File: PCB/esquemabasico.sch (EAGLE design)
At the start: 10 parts

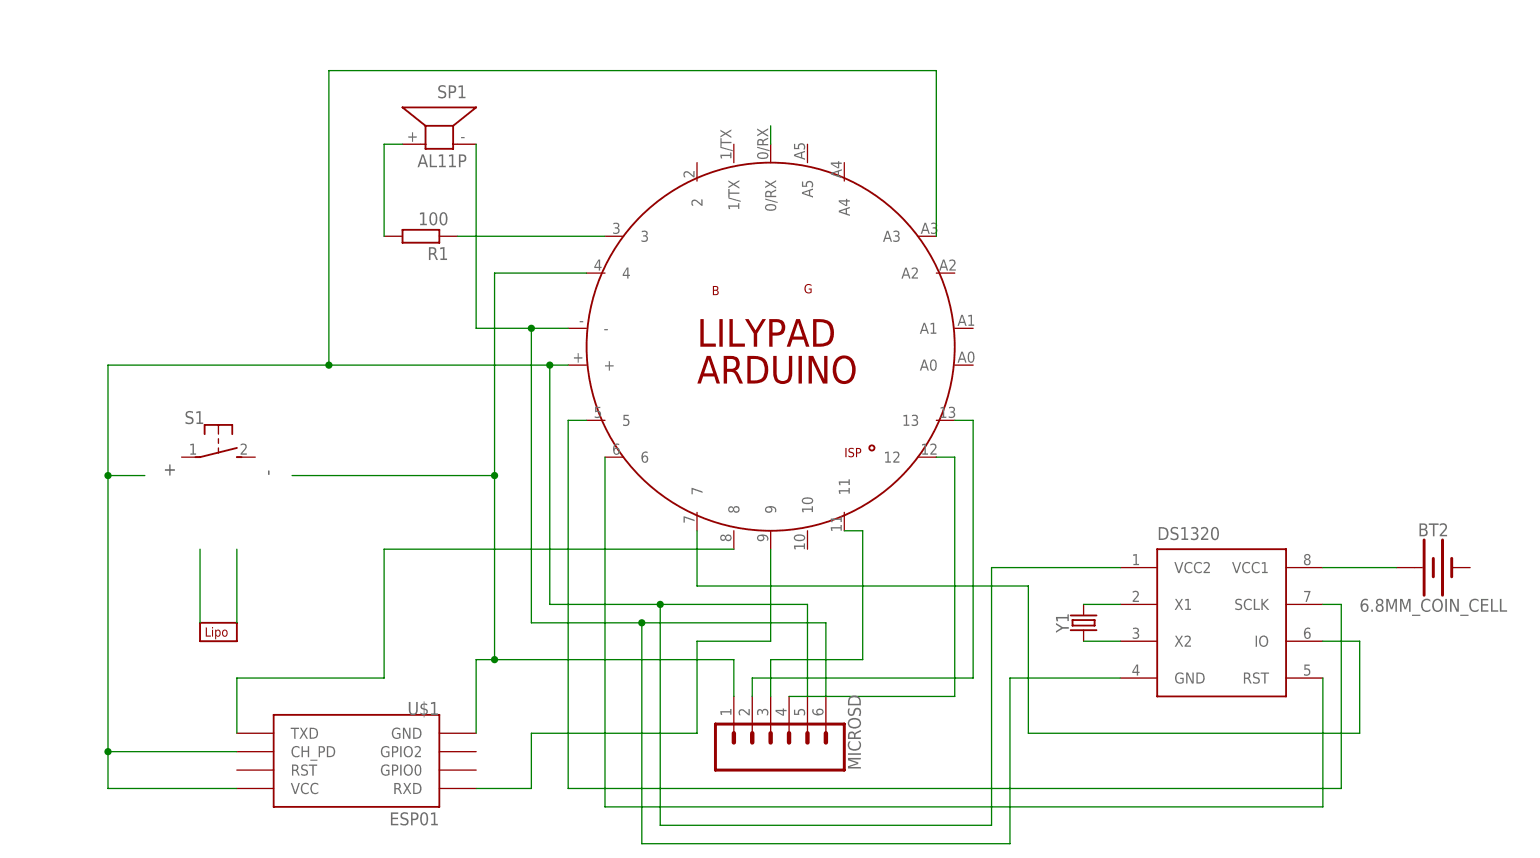
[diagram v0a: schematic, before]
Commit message: Cambios Finales PCB
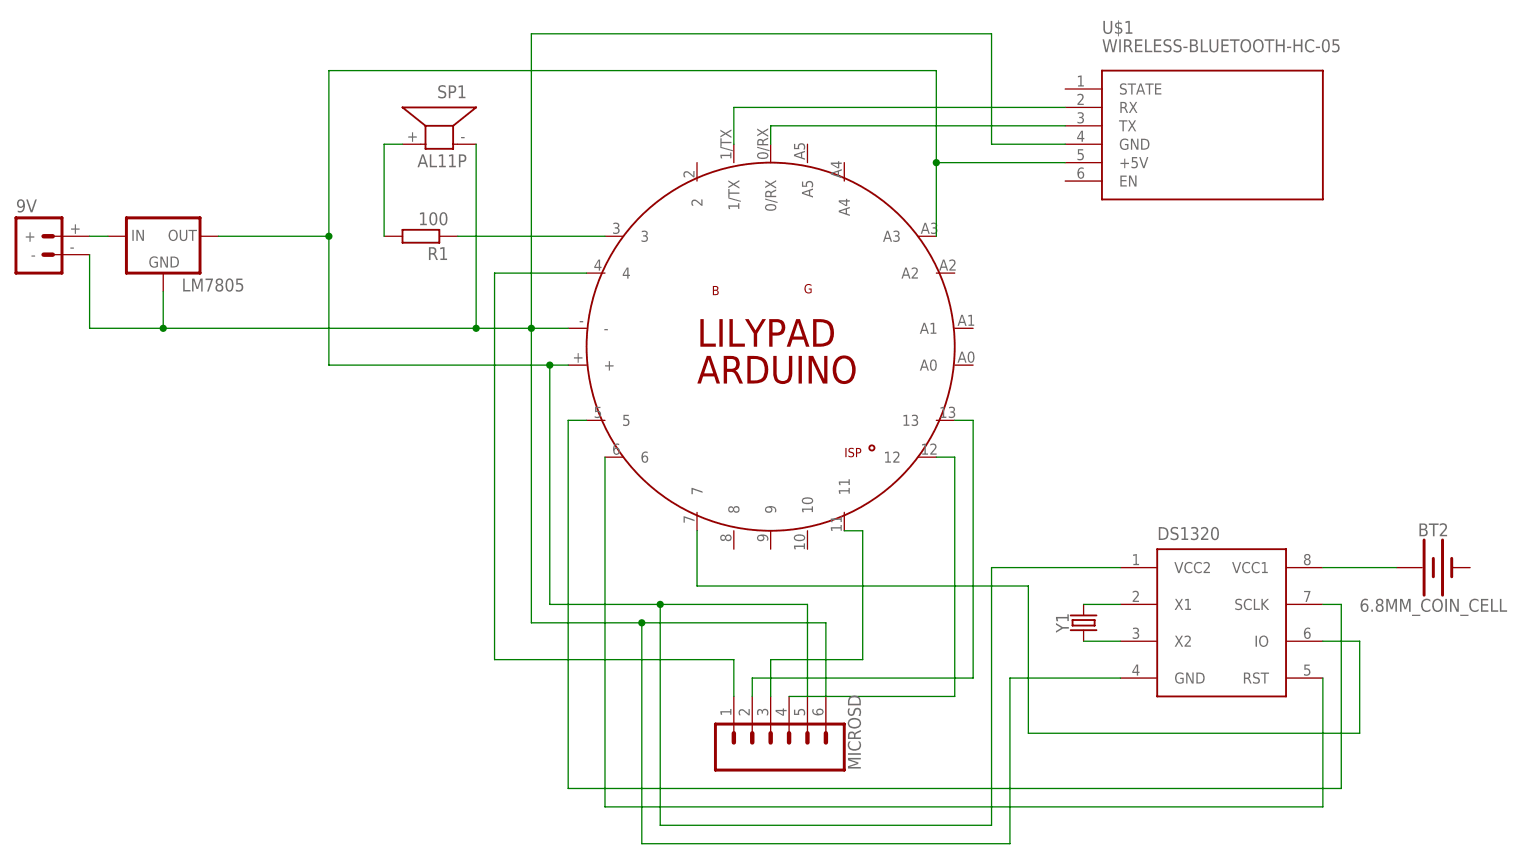
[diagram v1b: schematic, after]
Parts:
- removed BT1: LIPO-OUTLINE1100, SparkFun-Batteries:LIPO-OUTLINE1100
- removed S1: (no value), switch-omron:31-XX
- added 9V: (no value), SparkFun-Connectors:BATTERY_CONN_DEANS
- added LM7805: (no value), SparkFun-IC-Power:V_REG_78XX-TO-220
- U$1: value ESP01 -> WIRELESS-BLUETOOTH-HC-05; device esp8266:ESP01 -> diy-modules:WIRELESS-BLUETOOTH-HC-05
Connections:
- removed net N$19: PCB1.9, U$1.RXD
- new net N$2: 9V.+, LM7805.IN
- new net N$6: PCB1.1/TX, U$1.RX
- net N$1: no longer U$1.GND
- net N$14: now also U$1.TX
- net N$17: now also U$1.GND; no longer PCB1.8, U$1.TXD
- net N$3: now also LM7805.OUT, U$1.+5V; no longer U$1.CH_PD, U$1.VCC
- net N$5: now also 9V.-, LM7805.GND
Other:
- note removed: "+"
- note removed: "-"
- note removed: "Lilypad Simple Power"
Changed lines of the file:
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@@
 <part name="SP1" library="buzzer" library_urn="urn:adsk.eagle:library:113" deviceset="AL11P" device="" package3d_urn="urn:adsk.eagle:package:5308/1"/>
 <part name="R1" library="rcl" library_urn="urn:adsk.eagle:library:334" deviceset="R-EU_" device="0309/12" package3d_urn="urn:adsk.eagle:package:23571/1" value="100"/>
-<part name="BT1" library="SparkFun-Batteries" deviceset="LIPO-OUTLINE" device="1100"/>
-<part name="S1" library="switch-omron" library_urn="urn:adsk.eagle:library:377" deviceset="31-XX" device="" package3d_urn="urn:adsk.eagle:package:27487/1"/>
 <part name="DS1320" library="ltc1440_lt1529_ds1302" deviceset="DS1302" device=""/>
 <part name="BT2" library="SparkFun-Batteries" deviceset="BATTERY" device="-6.8MM_SMD" value="6.8MM_COIN_CELL"/>
 <part name="Y1" library="SparkFun-Clocks" deviceset="CRYSTAL" device="PTH-2X6"/>
-<part name="U$1" library="esp8266" deviceset="ESP01" device=""/>
+<part name="LM7805" library="SparkFun-IC-Power" deviceset="V_REG_78XX" device="-TO-220"/>
+<part name="9V" library="SparkFun-Connectors" deviceset="BATTERY_CONN" device="_DEANS"/>
+<part name="U$1" library="diy-modules" deviceset="WIRELESS-BLUETOOTH-HC-05" device=""/>
 </parts>
 <sheets>
 <sheet>
 <plain>
-<circle x="-12.7" y="25.4" radius="10.77630625" width="0.254" layer="133"/>
-<text x="-20.32" y="25.4" size="1.778" layer="97">+</text>
-<text x="-5.08" y="25.4" size="1.778" layer="97" rot="R90">-</text>
-<polygon width="0.254" layer="133" spacing="0.254" pour="hatch">
-<vertex x="-15.24" y="38.1"/>
-<vertex x="-15.24" y="35.56"/>
-<vertex x="-10.16" y="35.56"/>
-<vertex x="-10.16" y="38.1"/>
-</polygon>
-<text x="0" y="20.32" size="1.778" layer="133" rot="R180">Lilypad Simple Power</text>
 </plain>
 <instances>
@@
 <attribute name="VALUE" x="19.05" y="61.722" size="1.778" layer="96" rot="R180"/>
 </instance>
-<instance part="BT1" gate="G$1" x="-15.24" y="2.54" smashed="yes"/>
-<instance part="S1" gate="1" x="-12.7" y="27.94" smashed="yes" rot="R270">
-<attribute name="NAME" x="-14.605" y="34.29" size="1.778" layer="95" rot="R180"/>
-<attribute name="VALUE" x="-9.525" y="31.75" size="1.778" layer="96"/>
-</instance>
 <instance part="DS1320" gate="G$1" x="124.46" y="5.08" smashed="yes">
 <attribute name="NAME" x="116.84" y="16.51" size="1.778" layer="95"/>
@@
 <attribute name="VALUE" x="108.712" y="5.08" size="1.778" layer="96" font="vector" rot="R90" align="top-center"/>
 </instance>
-<instance part="U$1" gate="G$1" x="5.08" y="-17.78" smashed="yes" rot="MR0">
-<attribute name="NAME" x="17.78" y="-7.62" size="1.778" layer="95" rot="MR0"/>
-<attribute name="VALUE" x="17.78" y="-22.86" size="1.778" layer="95" rot="MR0"/>
+<instance part="LM7805" gate="G$1" x="-20.32" y="58.42" smashed="yes">
+<attribute name="NAME" x="-17.78" y="50.8" size="1.778" layer="95"/>
+<attribute name="VALUE" x="-17.78" y="48.26" size="1.778" layer="96"/>
+</instance>
+<instance part="9V" gate="G$1" x="-38.1" y="58.42" smashed="yes">
+<attribute name="VALUE" x="-40.64" y="50.8" size="1.778" layer="96" font="vector"/>
+<attribute name="NAME" x="-40.64" y="61.722" size="1.778" layer="95" font="vector"/>
+</instance>
+<instance part="U$1" gate="G$1" x="124.46" y="73.66" smashed="yes">
+<attribute name="NAME" x="109.22" y="86.36" size="1.778" layer="95"/>
+<attribute name="VALUE" x="109.22" y="83.82" size="1.778" layer="96"/>
 </instance>
 </instances>
@@
 <pinref part="PCB1" gate="G$1" pin="0/RX"/>
 <wire x1="63.5" y1="73.66" x2="63.5" y2="71.12" width="0.1524" layer="91"/>
+<pinref part="U$1" gate="G$1" pin="TX"/>
+<wire x1="63.5" y1="73.66" x2="104.14" y2="73.66" width="0.1524" layer="91"/>
 </segment>
 </net>
@@
 <pinref part="PCB1" gate="G$1" pin="4"/>
 <wire x1="38.1" y1="53.34" x2="25.4" y2="53.34" width="0.1524" layer="91"/>
-<wire x1="25.4" y1="53.34" x2="25.4" y2="25.4" width="0.1524" layer="91"/>
-<wire x1="25.4" y1="25.4" x2="25.4" y2="0" width="0.1524" layer="91"/>
+<wire x1="25.4" y1="53.34" x2="25.4" y2="0" width="0.1524" layer="91"/>
 <wire x1="25.4" y1="0" x2="58.42" y2="0" width="0.1524" layer="91"/>
 <pinref part="MICROSD" gate="G$1" pin="1"/>
 <wire x1="58.42" y1="0" x2="58.42" y2="-5.08" width="0.1524" layer="91"/>
-<wire x1="-2.54" y1="25.4" x2="25.4" y2="25.4" width="0.1524" layer="91"/>
-<junction x="25.4" y="25.4"/>
-<pinref part="U$1" gate="G$1" pin="GND"/>
-<wire x1="22.86" y1="-10.16" x2="22.86" y2="0" width="0.1524" layer="91"/>
-<wire x1="22.86" y1="0" x2="25.4" y2="0" width="0.1524" layer="91"/>
-<junction x="25.4" y="0"/>
 </segment>
 </net>
@@
 <wire x1="33.02" y1="40.64" x2="2.54" y2="40.64" width="0.1524" layer="91"/>
 <junction x="33.02" y="40.64"/>
-<wire x1="2.54" y1="40.64" x2="-27.94" y2="40.64" width="0.1524" layer="91"/>
-<wire x1="-27.94" y1="40.64" x2="-27.94" y2="25.4" width="0.1524" layer="91"/>
-<wire x1="-27.94" y1="25.4" x2="-22.86" y2="25.4" width="0.1524" layer="91"/>
-<wire x1="2.54" y1="40.64" x2="2.54" y2="81.28" width="0.1524" layer="91"/>
-<junction x="2.54" y="40.64"/>
+<wire x1="2.54" y1="40.64" x2="2.54" y2="58.42" width="0.1524" layer="91"/>
 <pinref part="PCB1" gate="G$1" pin="A3"/>
+<wire x1="2.54" y1="58.42" x2="2.54" y2="81.28" width="0.1524" layer="91"/>
 <wire x1="2.54" y1="81.28" x2="86.36" y2="81.28" width="0.1524" layer="91"/>
-<wire x1="86.36" y1="81.28" x2="86.36" y2="58.42" width="0.1524" layer="91"/>
+<wire x1="86.36" y1="81.28" x2="86.36" y2="68.58" width="0.1524" layer="91"/>
 <pinref part="DS1320" gate="G$1" pin="VCC2"/>
+<wire x1="86.36" y1="68.58" x2="86.36" y2="58.42" width="0.1524" layer="91"/>
 <wire x1="111.76" y1="12.7" x2="93.98" y2="12.7" width="0.1524" layer="91"/>
 <wire x1="93.98" y1="12.7" x2="93.98" y2="-22.86" width="0.1524" layer="91"/>
@@
 <wire x1="48.26" y1="-22.86" x2="48.26" y2="7.62" width="0.1524" layer="91"/>
 <junction x="48.26" y="7.62"/>
-<pinref part="U$1" gate="G$1" pin="CH_PD"/>
-<wire x1="-27.94" y1="25.4" x2="-27.94" y2="-12.7" width="0.1524" layer="91"/>
-<wire x1="-27.94" y1="-12.7" x2="-10.16" y2="-12.7" width="0.1524" layer="91"/>
-<junction x="-27.94" y="25.4"/>
-<pinref part="U$1" gate="G$1" pin="VCC"/>
-<wire x1="-27.94" y1="-12.7" x2="-27.94" y2="-17.78" width="0.1524" layer="91"/>
-<wire x1="-27.94" y1="-17.78" x2="-10.16" y2="-17.78" width="0.1524" layer="91"/>
-<junction x="-27.94" y="-12.7"/>
+<pinref part="LM7805" gate="G$1" pin="OUT"/>
+<wire x1="-12.7" y1="58.42" x2="2.54" y2="58.42" width="0.1524" layer="91"/>
+<junction x="2.54" y="58.42"/>
+<pinref part="U$1" gate="G$1" pin="+5V"/>
+<wire x1="104.14" y1="68.58" x2="86.36" y2="68.58" width="0.1524" layer="91"/>
+<junction x="86.36" y="68.58"/>
 </segment>
 </net>
@@
 <wire x1="45.72" y1="-25.4" x2="45.72" y2="5.08" width="0.1524" layer="91"/>
 <junction x="45.72" y="5.08"/>
-</segment>
-</net>
-<net name="N$2" class="0">
-<segment>
-<wire x1="-15.24" y1="5.08" x2="-15.24" y2="15.24" width="0.1524" layer="91"/>
-</segment>
-</net>
-<net name="N$6" class="0">
-<segment>
-<wire x1="-10.16" y1="5.08" x2="-10.16" y2="15.24" width="0.1524" layer="91"/>
+<wire x1="22.86" y1="45.72" x2="-20.32" y2="45.72" width="0.1524" layer="91"/>
+<junction x="22.86" y="45.72"/>
+<pinref part="LM7805" gate="G$1" pin="GND"/>
+<wire x1="-20.32" y1="45.72" x2="-20.32" y2="50.8" width="0.1524" layer="91"/>
+<pinref part="9V" gate="G$1" pin="-"/>
+<wire x1="-30.48" y1="55.88" x2="-30.48" y2="45.72" width="0.1524" layer="91"/>
+<wire x1="-30.48" y1="45.72" x2="-20.32" y2="45.72" width="0.1524" layer="91"/>
+<junction x="-20.32" y="45.72"/>
 </segment>
 </net>
@@
 </segment>
 </net>
+<net name="N$2" class="0">
+<segment>
+<pinref part="9V" gate="G$1" pin="+"/>
+<pinref part="LM7805" gate="G$1" pin="IN"/>
+<wire x1="-30.48" y1="58.42" x2="-27.94" y2="58.42" width="0.1524" layer="91"/>
+</segment>
+</net>
+<net name="N$6" class="0">
+<segment>
+<pinref part="U$1" gate="G$1" pin="RX"/>
+<pinref part="PCB1" gate="G$1" pin="1/TX"/>
+<wire x1="104.14" y1="76.2" x2="58.42" y2="76.2" width="0.1524" layer="91"/>
+<wire x1="58.42" y1="76.2" x2="58.42" y2="71.12" width="0.1524" layer="91"/>
+</segment>
+</net>
 <net name="N$17" class="0">
 <segment>
-<pinref part="U$1" gate="G$1" pin="TXD"/>
-<wire x1="-10.16" y1="-10.16" x2="-10.16" y2="-2.54" width="0.1524" layer="91"/>
-<wire x1="-10.16" y1="-2.54" x2="10.16" y2="-2.54" width="0.1524" layer="91"/>
-<wire x1="10.16" y1="-2.54" x2="10.16" y2="15.24" width="0.1524" layer="91"/>
-<pinref part="PCB1" gate="G$1" pin="8"/>
-<wire x1="10.16" y1="15.24" x2="58.42" y2="15.24" width="0.1524" layer="91"/>
-</segment>
-</net>
-<net name="N$19" class="0">
-<segment>
-<pinref part="U$1" gate="G$1" pin="RXD"/>
-<wire x1="22.86" y1="-17.78" x2="30.48" y2="-17.78" width="0.1524" layer="91"/>
-<wire x1="30.48" y1="-17.78" x2="30.48" y2="-10.16" width="0.1524" layer="91"/>
-<wire x1="30.48" y1="-10.16" x2="53.34" y2="-10.16" width="0.1524" layer="91"/>
-<wire x1="53.34" y1="-10.16" x2="53.34" y2="2.54" width="0.1524" layer="91"/>
-<wire x1="53.34" y1="2.54" x2="63.5" y2="2.54" width="0.1524" layer="91"/>
-<pinref part="PCB1" gate="G$1" pin="9"/>
-<wire x1="63.5" y1="2.54" x2="63.5" y2="15.24" width="0.1524" layer="91"/>
-</segment>
-</net>
+<pinref part="U$1" gate="G$1" pin="GND"/>
+<wire x1="104.14" y1="71.12" x2="93.98" y2="71.12" width="0.1524" layer="91"/>
+<wire x1="93.98" y1="71.12" x2="93.98" y2="86.36" width="0.1524" layer="91"/>
+<wire x1="93.98" y1="86.36" x2="30.48" y2="86.36" width="0.1524" layer="91"/>
+<wire x1="30.48" y1="86.36" x2="30.48" y2="45.72" width="0.1524" layer="91"/>
+</segment>
+</net>
